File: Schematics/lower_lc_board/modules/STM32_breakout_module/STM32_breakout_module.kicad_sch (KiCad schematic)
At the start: 42 parts, among them J2 SWD_CONN, J3 USB_C_CONN, SW1 SW_STM_RESET, SW2 SW_STM_BOOT_MODE, U5 STM32F103CBT6, U6 W25Q128JVS, U7 ISO1044BDR, U8 CP2102N-Axx-xQFN28, Y1 X322516MMB4SI

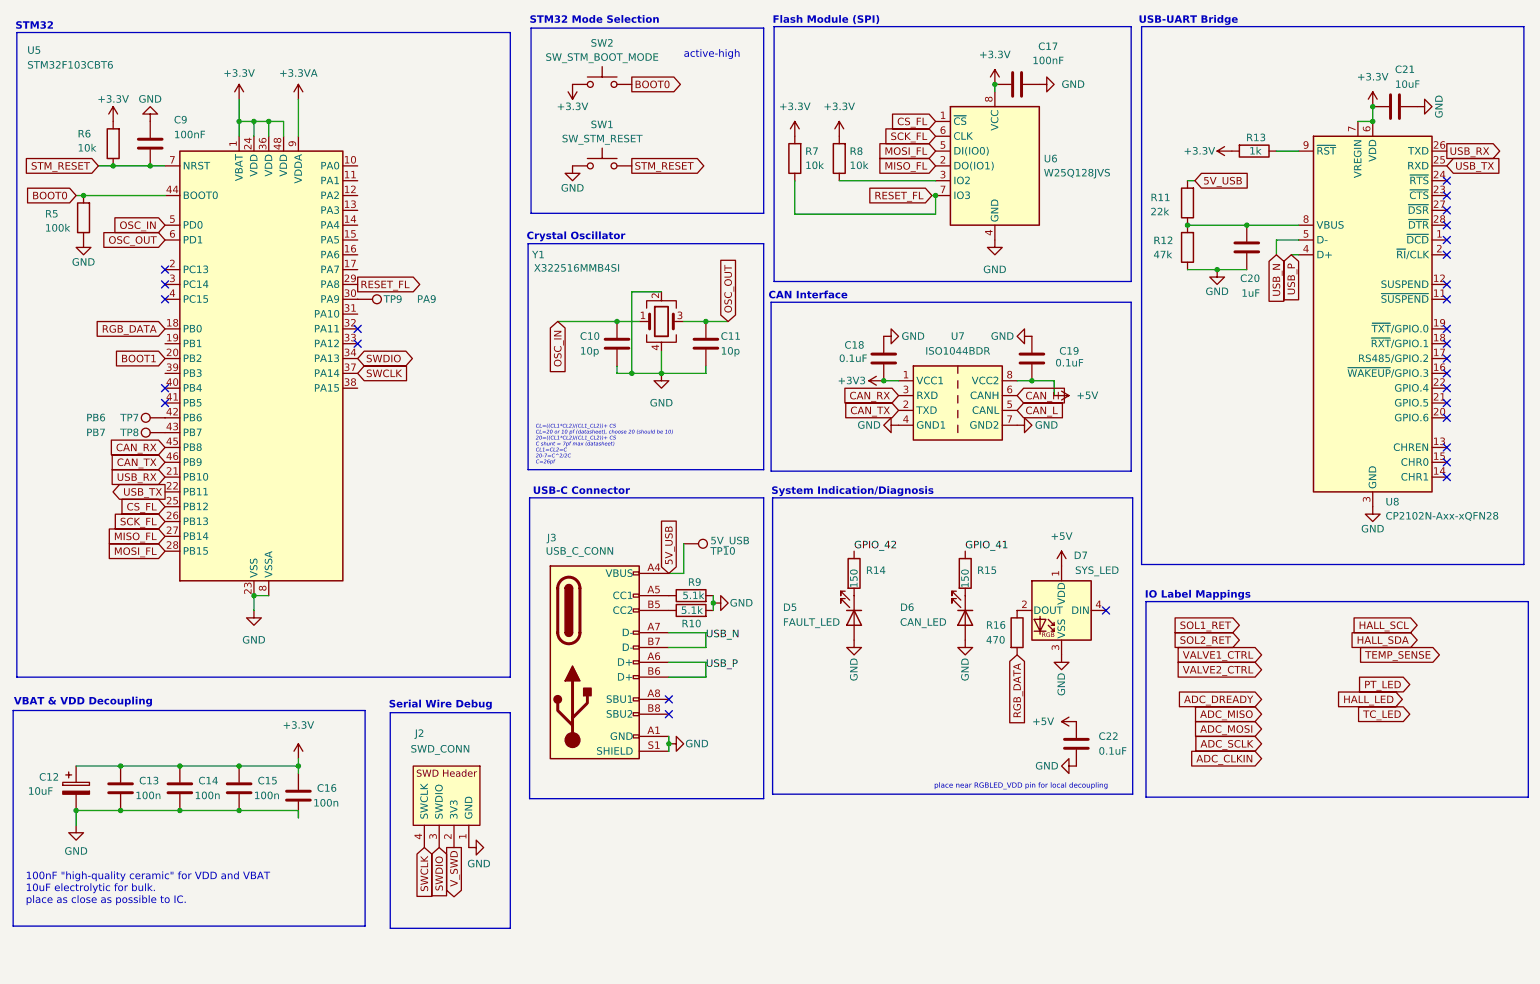
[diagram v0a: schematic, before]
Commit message: pin assignments verified
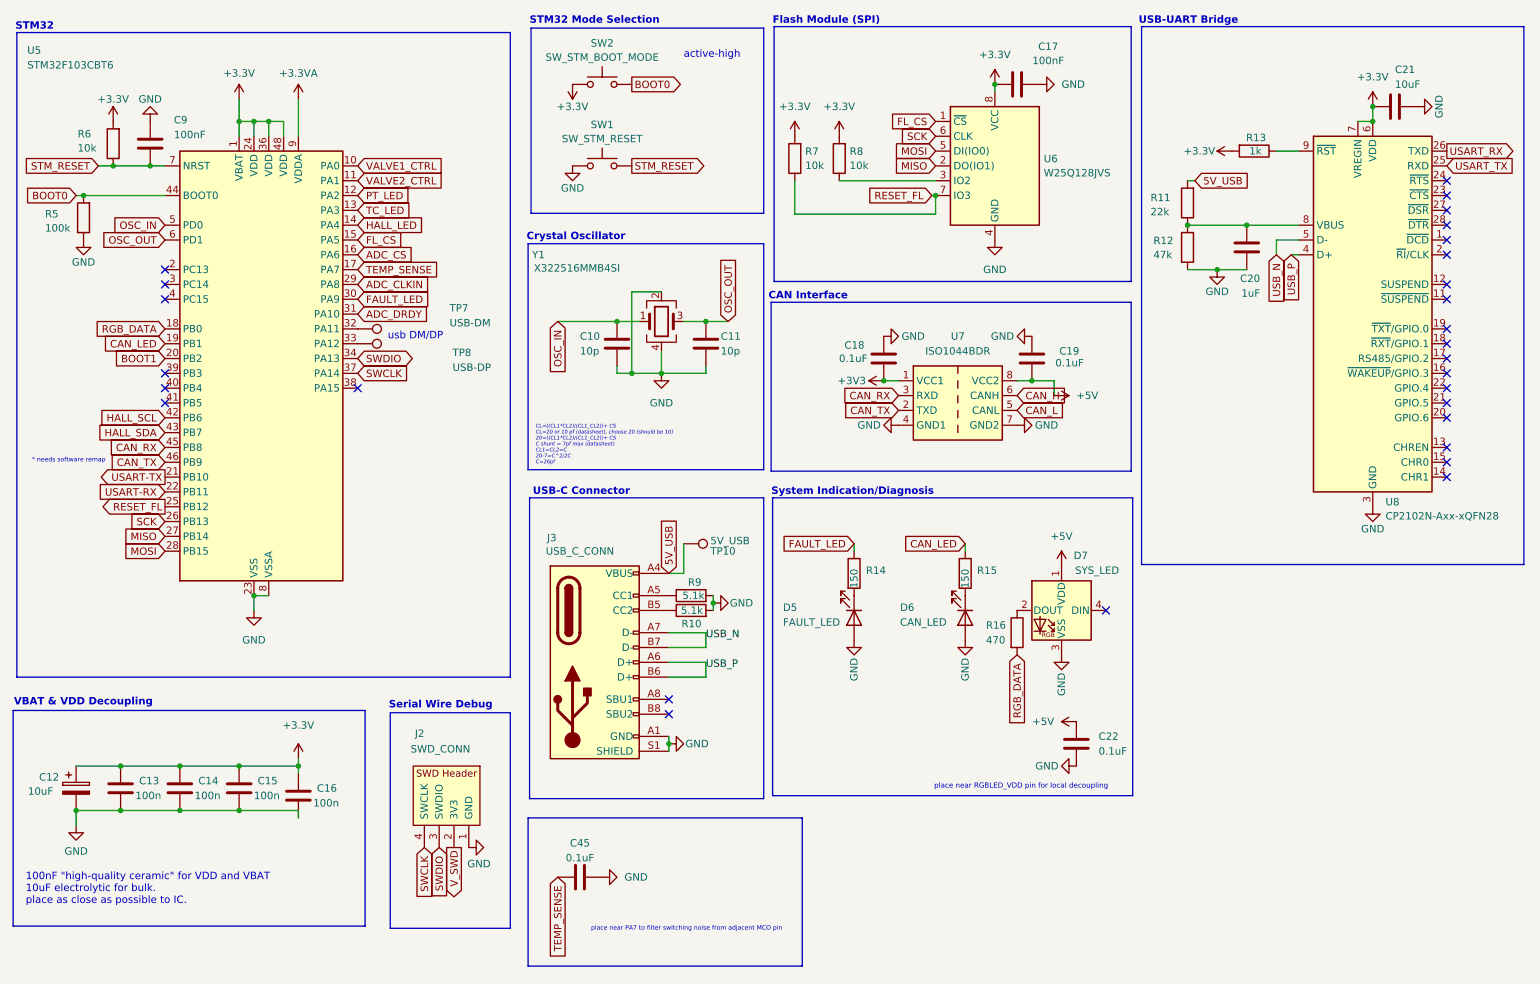
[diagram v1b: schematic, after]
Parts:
- removed TP9: PA9, TestPoint:TestPoint_Pad_1.5x1.5mm, symbol Connector:TestPoint
- added C45: 0.1uF, Capacitor_SMD:C_0805_2012Metric, symbol Device:C
- TP7: value PB6 -> USB-DM; footprint TestPoint:TestPoint_Pad_1.5x1.5mm -> TestPoint:TestPoint_Pad_D1.5mm; now in the parts list
- TP8: value PB7 -> USB-DP; footprint TestPoint:TestPoint_Pad_1.5x1.5mm -> TestPoint:TestPoint_Pad_D1.5mm; now in the parts list
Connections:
- net GPIO_41 is gone; now on net CAN_LED: R15.1
- net GPIO_42 is gone; now on net FAULT_LED: R14.1
- net ADC_CLKIN: now also U5.29 (PA8)
- net GND: now also C45.1
- net HALL_LED: now also U5.14 (PA4)
- net HALL_SCL: now also U5.42 (PB6)
- net HALL_SDA: now also U5.43 (PB7)
- net PT_LED: now also U5.12 (PA2)
- net RESET_FL: now also U5.25 (PB12); no longer U5.29 (PA8)
- net TC_LED: now also U5.13 (PA3)
- net TEMP_SENSE: now also U5.17 (PA7), C45.2
- net VALVE1_CTRL: now also U5.10 (PA0)
- net VALVE2_CTRL: now also U5.11 (PA1)
- net at TP7.1: now also U5.32 (PA11); no longer U5.42 (PB6)
- net FAULT_LED: now reaches U5.30 (PA9)
- net at TP8.1: now also U5.33 (PA12); no longer U5.43 (PB7)
- net FL_CS: now reaches U5.15 (PA5)
- net FL_CS: now also U6.1 (~{CS})
- net ADC_CS: now reaches U5.16 (PA6)
- net CAN_LED: now reaches U5.19 (PB1)
- net ADC_DRDY: now reaches U5.31 (PA10)
- removed net CS_FL: U5.25 (PB12), U6.1 (~{CS})
- net MISO_FL renamed MISO
- net MOSI_FL renamed MOSI
- net SCK_FL renamed SCK
- net USB_RX renamed USART-TX
- net USART-TX: no longer U8.26 (TXD)
- net USB_TX renamed USART-RX
- net USART-RX: no longer U8.25 (RXD)
- new net USART_RX: U8.26 (TXD)
- new net USART_TX: U8.25 (RXD)
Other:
- note added: "* needs software remap"
- note added: "place near PA7 to filter switching noise from adjacent MCO pin"
- note added: "usb DM/DP"
- note removed: "IO Label Mappings"
